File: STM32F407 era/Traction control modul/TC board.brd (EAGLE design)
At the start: 79.7 x 100 mm, 49 parts, among them IC1 74HC14D, IC2 lm2575, IC3 74AC08D, IC4 74AC04D, J1 CON1, U1 MAX13052ESA+, U2 MAX232AEWE+, X1 057-006-1

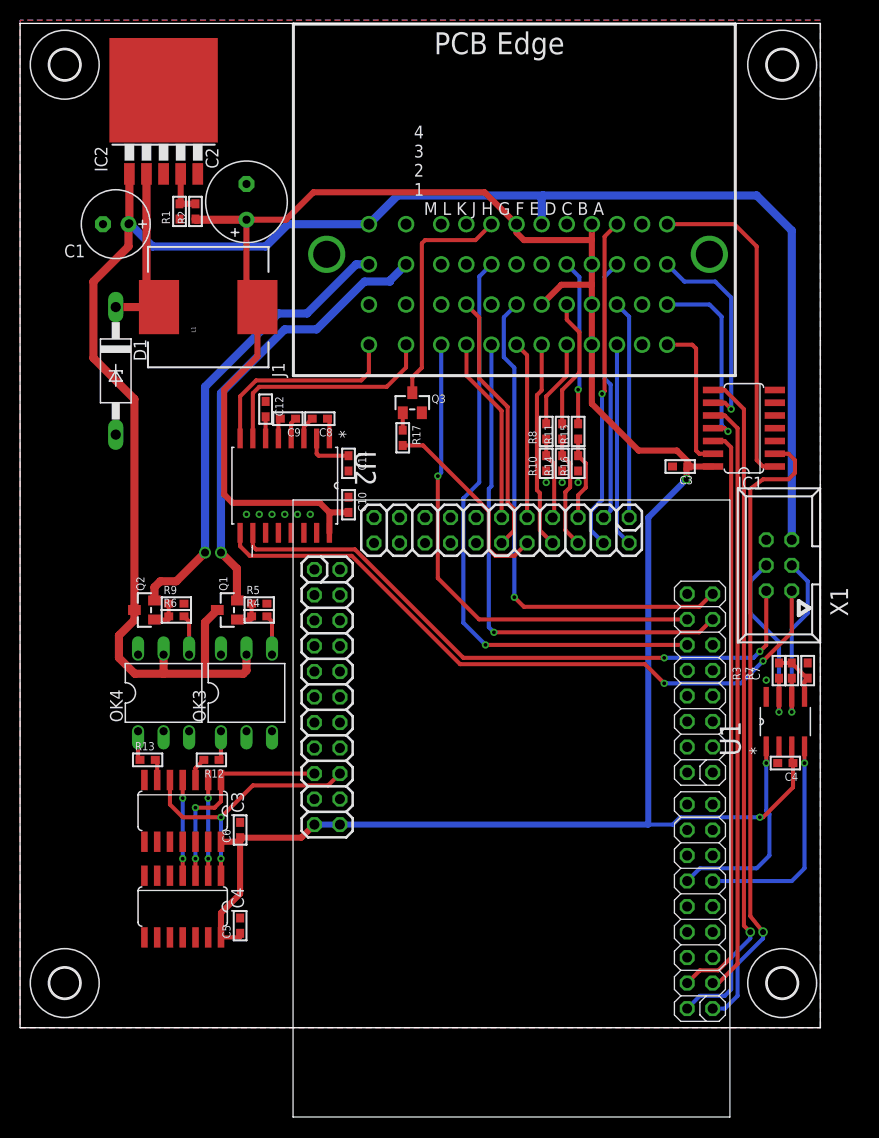
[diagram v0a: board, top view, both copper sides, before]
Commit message: moved outfaced boards to new folder
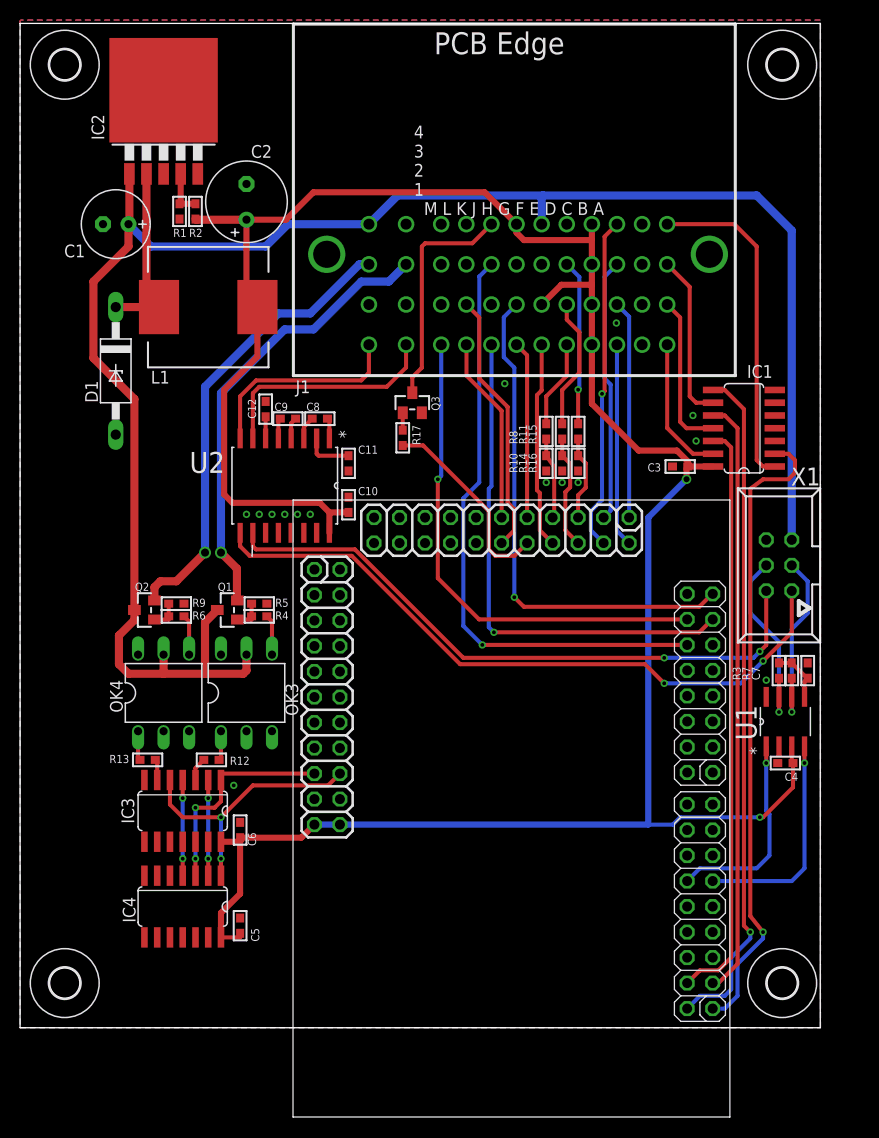
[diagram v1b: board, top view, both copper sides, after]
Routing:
- net N$3: track 20.9 -> 16.7 mm, vias 1 -> 0
- net N$6: track 19.2 -> 15.8 mm, vias 1 -> 0
- net N$4: track 15.0 -> 13.9 mm
- net 12V: track 180.0 -> 180.3 mm, vias 1 -> 0
